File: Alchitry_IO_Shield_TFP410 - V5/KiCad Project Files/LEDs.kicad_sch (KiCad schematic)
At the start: 52 parts, among them Q1 Q_PMOS_SGD, Q2 Q_PMOS_SGD, Q3 Q_PMOS_SGD, Q4 Q_PMOS_SGD, SW1 SWL3, SW10 SW_DIP_x08, SW2 SWL1, SW3 SWL2, SW4 SWL4, SW5 SWR3, SW6 SWR1, SW7 SWR2, SW8 SWR3, SW9 SW_DIP_x08

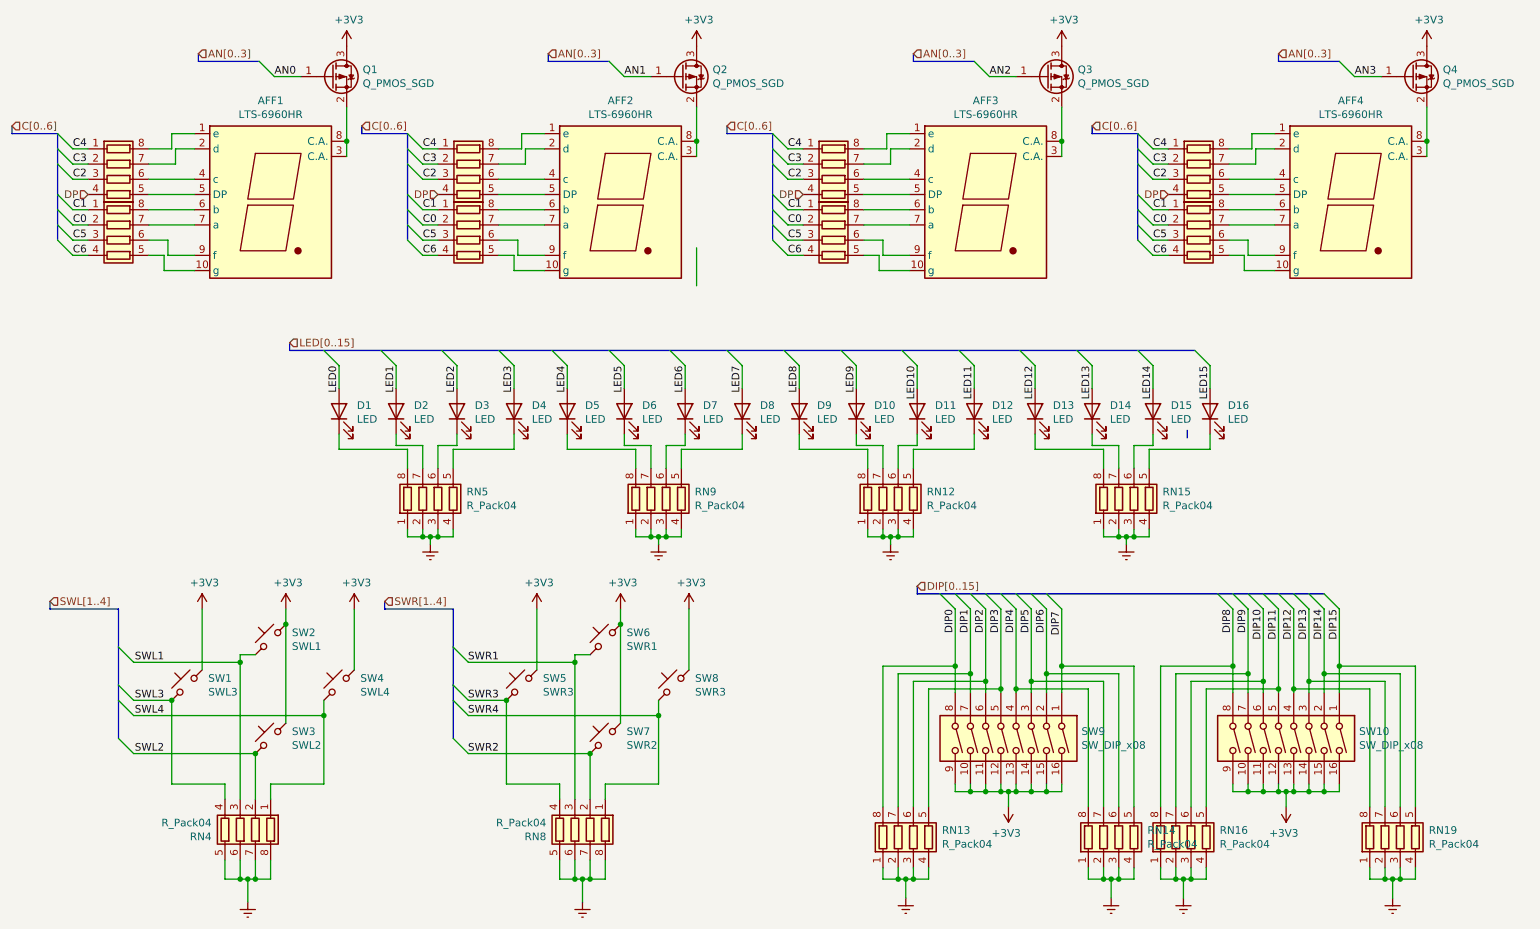
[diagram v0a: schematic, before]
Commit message: started new shield
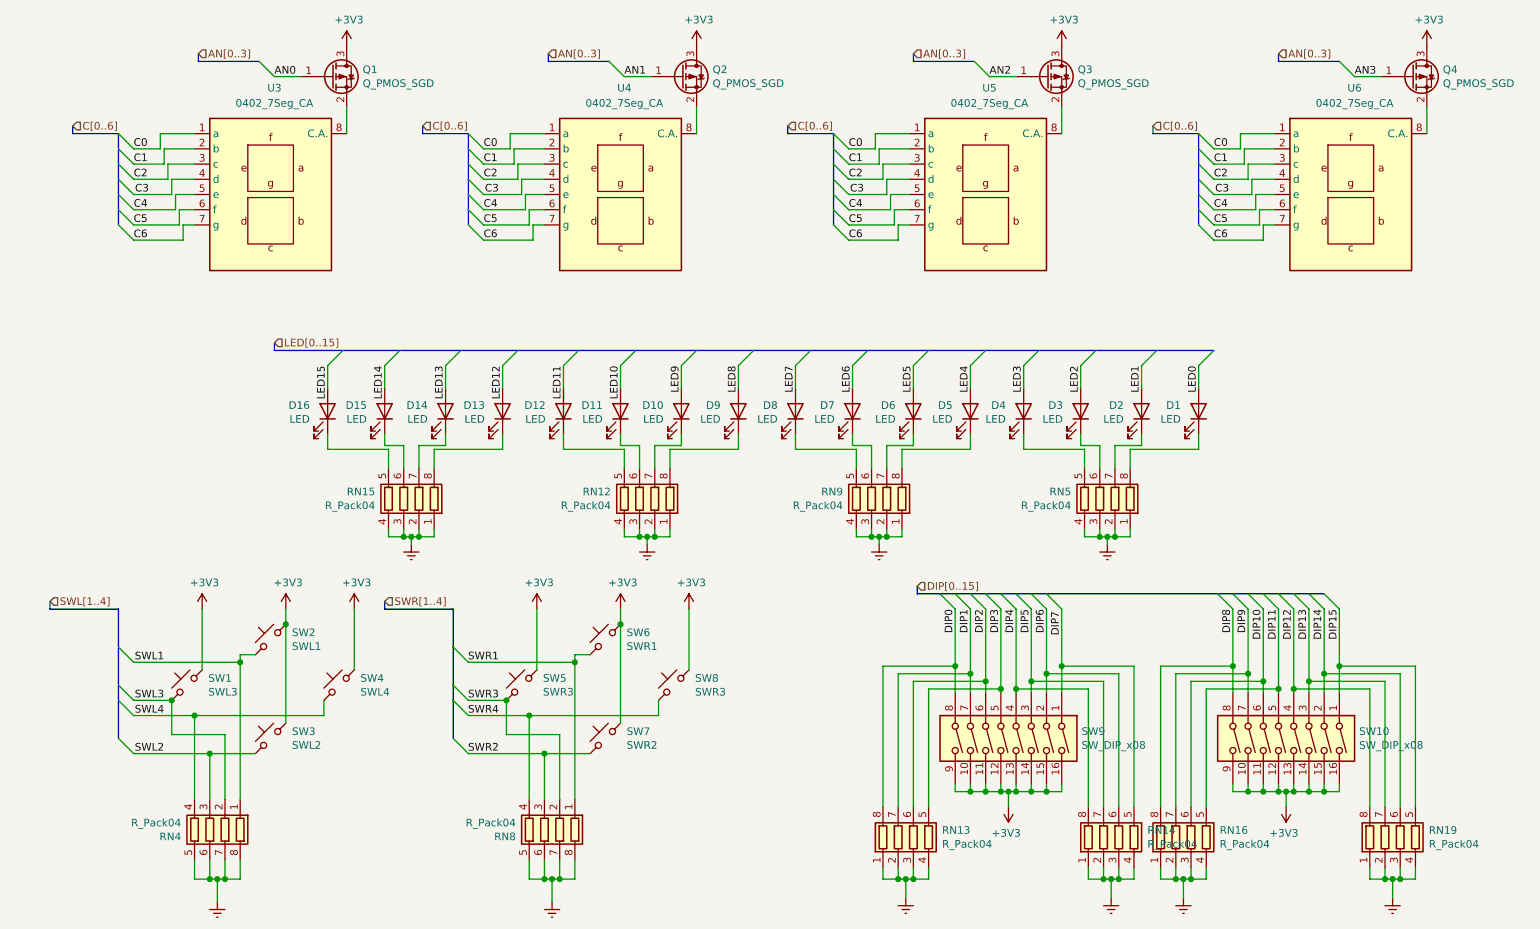
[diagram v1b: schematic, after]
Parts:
- removed AFF1, AFF2, AFF3, AFF4: LTS-6960HR, Display_7Segment:KCSC02-105, symbol 7_Segment_LTS6780:LTS-6960HR
- removed RN10, RN11, RN17, RN18, RN2, RN3, RN6, RN7: R_Pack04, Resistor_SMD:R_Array_Convex_4x0603, symbol Device:R_Pack04
- added U3, U4, U5, U6: 0402_7Seg_CA, Custom_LEDs:0402_7Seg_CA_W_Res, symbol Custom_LEDs:0402_7Seg_CA_W_Res
- D1, D10, D11, D12, D13, D14, D15, D16, D2, D3, D4, D5, D6, D7, D8, D9: footprint LED_SMD:LED_0603_1608Metric_Pad1.05x0.95mm_HandSolder -> LED_SMD:LED_0402_1005Metric
- SW1, SW2, SW3, SW4, SW5, SW6, SW7, SW8: footprint Button_Switch_SMD:SW_SPST_TL3342 -> Custom_Buttons:Korean Hroparts Elec K2-1177SR
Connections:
- net C0: now also U3.1 (a), U4.1 (a), U5.1 (a), U6.1 (a)
- net C1: now also U3.2 (b), U4.2 (b), U5.2 (b), U6.2 (b)
- net C2: now also U3.3 (c), U4.3 (c), U5.3 (c), U6.3 (c)
- net C3: now also U3.4 (d), U4.4 (d), U5.4 (d), U6.4 (d)
- net C4: now also U3.5 (e), U4.5 (e), U5.5 (e), U6.5 (e)
- net C5: now also U3.6 (f), U4.6 (f), U5.6 (f), U6.6 (f)
- net C6: now also U3.7 (g), U4.7 (g), U5.7 (g), U6.7 (g)
- net SWL1: now also RN4.1 (R1.1); no longer RN4.3 (R3.1)
- net SWL2: now also RN4.3 (R3.1); no longer RN4.2 (R2.1)
- net SWL3: now also RN4.2 (R2.1); no longer RN4.4 (R4.1)
- net SWL4: now also RN4.4 (R4.1); no longer RN4.1 (R1.1)
- net SWR1: now also RN8.1 (R1.1); no longer RN8.3 (R3.1)
- net SWR2: now also RN8.3 (R3.1); no longer RN8.2 (R2.1)
- net SWR3: now also RN8.2 (R2.1); no longer RN8.4 (R4.1)
- net SWR4: now also RN8.4 (R4.1); no longer RN8.1 (R1.1)
- net at Q1.2 (S): now also U3.8 (C.A.)
- net at Q2.2 (S): now also U4.8 (C.A.)
- net at Q3.2 (S): now also U5.8 (C.A.)
- net at Q4.2 (S): now also U6.8 (C.A.)
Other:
- moved on the sheet: D1, D10, D11, D12, D13, D14, D15, D16, D2, D3, D4, D5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
